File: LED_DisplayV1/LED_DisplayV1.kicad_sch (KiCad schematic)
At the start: 10 parts, among them U1 A3144

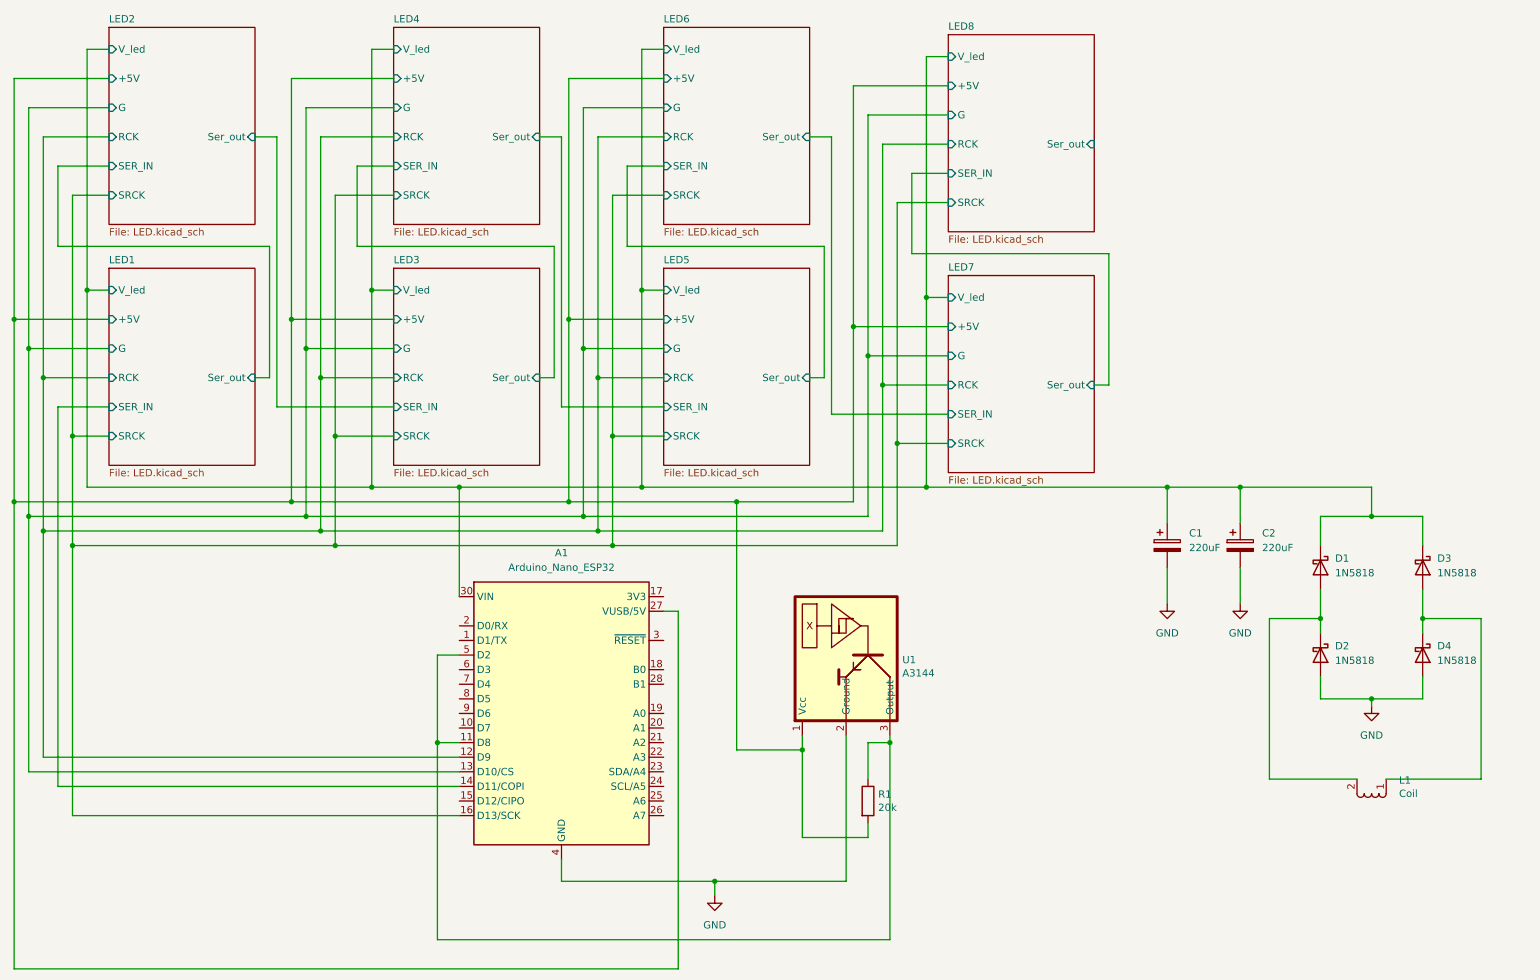
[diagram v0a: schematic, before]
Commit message: All_wired
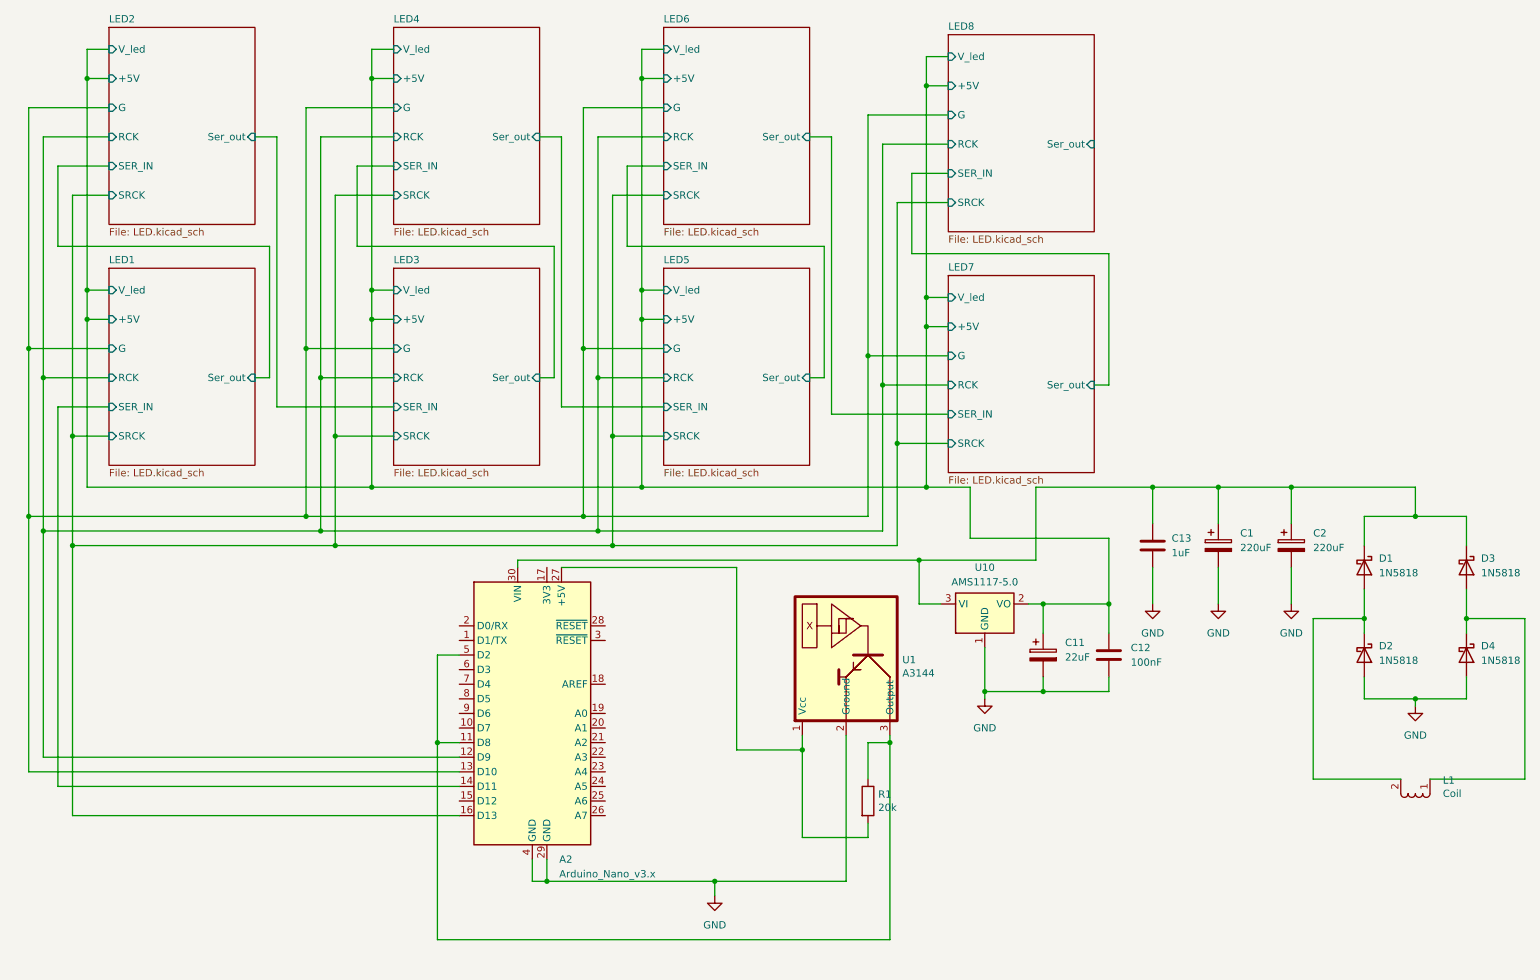
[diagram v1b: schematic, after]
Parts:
- removed A1: Arduino_Nano_ESP32, Module:Arduino_Nano, symbol MCU_Module:Arduino_Nano_ESP32
- added A2: Arduino_Nano_v3.x, Module:Arduino_Nano, symbol MCU_Module:Arduino_Nano_v3.x
- added C11: 22uF, Capacitor_Tantalum_SMD:CP_EIA-3528-12_Kemet-T_HandSolder, symbol Device:C_Polarized
- added C12: 100nF, Capacitor_SMD:C_0603_1608Metric_Pad1.08x0.95mm_HandSolder, symbol Device:C
- added C13: 1uF, Capacitor_SMD:C_0805_2012Metric_Pad1.18x1.45mm_HandSolder, symbol Device:C
- added U10: AMS1117-5.0, Package_TO_SOT_SMD:SOT-223-3_TabPin2, symbol Regulator_Linear:AMS1117-5.0
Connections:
- net GND: now also A2.29 (GND), A2.4 (GND), C11.2, C12.2, C13.2, U10.1 (GND)
- net LED1/+5V: now also C11.1, C12.1, U10.2 (VO); no longer R1.2, U1.1 (Vcc)
- net LED1/G: now also A2.13 (D10)
- net LED1/RCK: now also A2.12 (D9)
- net LED1/SER_IN: now also A2.14 (D11)
- net LED1/SRCK: now also A2.16 (D13)
- net at R1.1, U1.3 (Output): now also A2.11 (D8), A2.5 (D2)
- net LED1/V_led: no longer names the net of C1.1, C2.1, D1.1 (K), D3.1 (K)
- net LED1/V_led: now also A2.30 (VIN), C13.1, U10.3 (VI)
- new net: A2.27 (+5V), R1.2, U1.1 (Vcc)
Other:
- moved on the sheet: C1, C2, D1, D2, D3, D4, L1
